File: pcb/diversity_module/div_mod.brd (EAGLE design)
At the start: 40.6 x 29.5 mm, 13 parts, among them IC1 REG113, IC2 74AHC1G126DBV

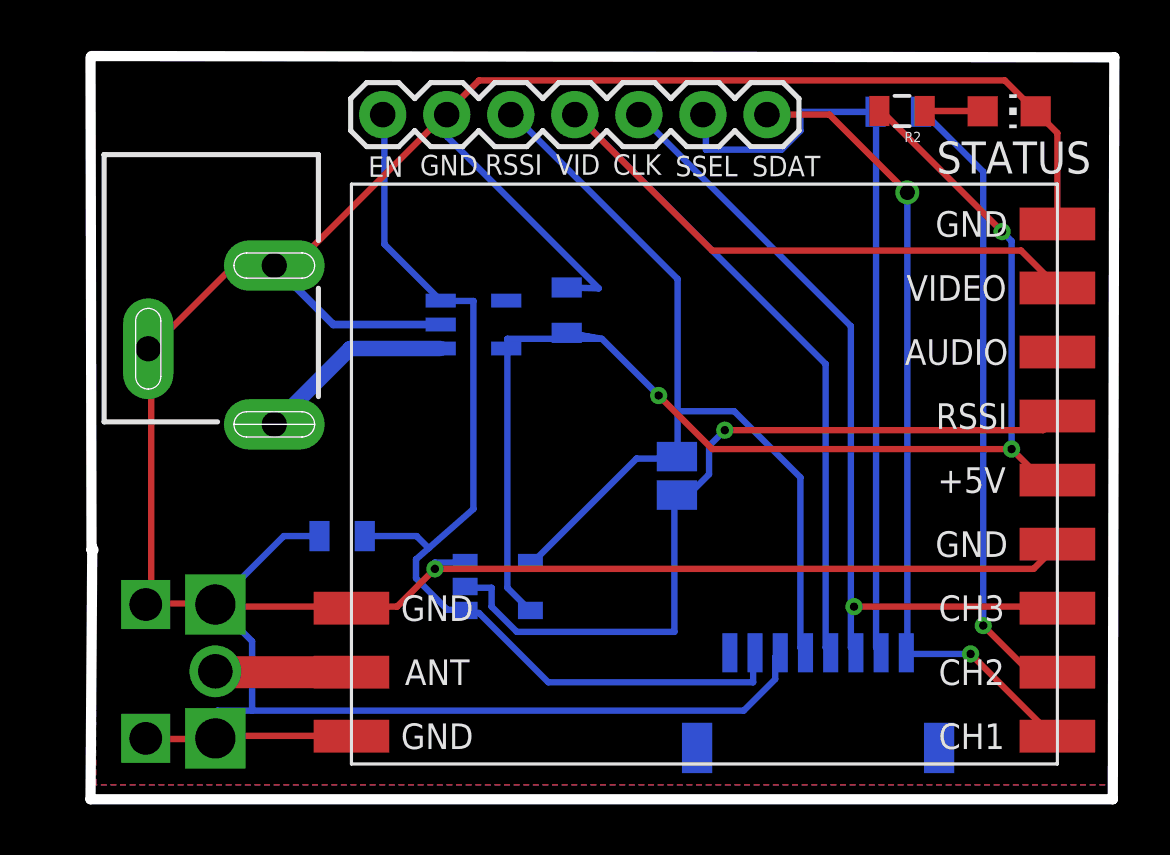
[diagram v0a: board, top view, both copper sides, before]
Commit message: diversity module v2.0
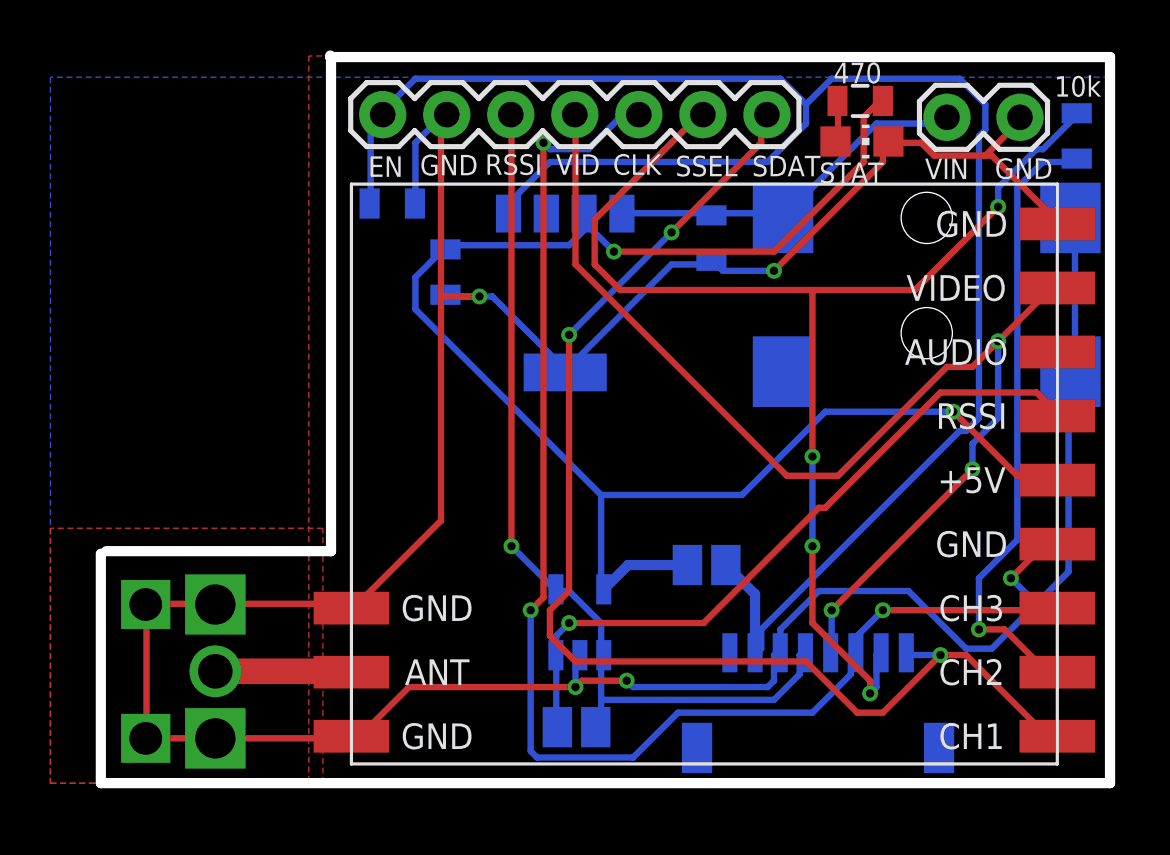
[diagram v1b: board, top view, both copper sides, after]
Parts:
- removed IC1: REG113, texas:SOT23-DBV
- removed IC2: 74AHC1G126DBV, 74xx-little-de:SOT23-5
- removed STATUS: (no value), led:CHIP-LED0805
- added C2: 1uf, SparkFun-Capacitors:0805
- added IC3: OPA336N, burr-brown:SOT23-5
- added JP2: (no value), SparkFun-Connectors:1X02_LOCK
- added SJ1: (no value), jumper:SJ
- added STAT: (no value), led:CHIP-LED0805
- added V1: LP38692P, lp38692:TO252-51
- C1: value 0.1uf -> 1uf
- JP1: value POWER_JACKSLT -> 5.5x2.1mm Barrel; device SparkFun-Connectors:POWER_JACK_SLOT -> SparkFun-Connectors:POWER_JACK_SMD
- moved JP1 24.0 mm to (34.8, 22.4), flipped to the bottom, turned to 270 degrees
- moved R3 13.3 mm to (13.6, 23.0), turned to 0 degrees
- moved SJ2 10.7 mm to (20.9, 2.22), turned to 180 degrees
- moved R1 7.14 mm to (40.7, 25.7), turned to 90 degrees
- moved C1 5.04 mm to (15.7, 20.3), turned to 270 degrees
- moved R2 1.71 mm to (32.1, 27.1), turned to 0 degrees
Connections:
- net 5V: now also IC3.5, SJ1.2, V1.OUT; no longer IC1.5, IC2.5
- net ENABLE: now also SJ1.1, V1.EN; no longer IC1.3, IC2.1
- net GND: now also C2.2, IC3.2, JP1.GND, JP1.P$4, JP2.1, STAT.C, V1.GND; no longer IC1.2, IC2.3, JP1.GND@1, JP1.GND@2, STATUS.C
- net N$2: now also STAT.A; no longer STATUS.A
- net RSSI_B: now also IC3.1, IC3.4; no longer IC2.4
- net RSSI_MOD: now also IC3.3; no longer IC2.2
- net VIN_UNREG: now also C2.1, JP1.VIN0, JP2.2, V1.IN; no longer IC1.1, JP1.PWR
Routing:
- net ENABLE: track 40.7 -> 73.6 mm
- net SPI_CLK: track 33.1 -> 53.0 mm, vias 1 -> 3
- net GND: track 155.5 -> 136.3 mm, vias 1 -> 5
- net SPI_SEL_B: track 30.8 -> 49.5 mm, vias 0 -> 4
- net SPI_DATA: track 32.5 -> 49.4 mm, vias 2 -> 3
- net 5V: track 53.6 -> 64.4 mm, vias 3 -> 2
- net VIN_UNREG: track 7.85 -> 14.9 mm
- net RSSI_MOD: track 32.6 -> 28.0 mm
- net RSSI_B: track 36.9 -> 35.7 mm, vias 0 -> 1
- net RXVIDOUT2: track 47.6 -> 46.9 mm, vias 0 -> 3
- net N$2: track 2.30 -> 1.64 mm
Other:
- board size 40.6 x 29.5 mm -> 40 x 28.9 mm
- board text added: "10k"
- board text added: "470"
- board text added: "VIN"
- board text added: "power"
